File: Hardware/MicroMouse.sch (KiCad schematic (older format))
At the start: 74 parts, among them J1 TSW-106-25-S-S-RA, J2 B2B-PH-K-S(LF)(SN), J3 Conn_01x04_Male, J4 B5B-XH-A(LF)(SN), J5 B5B-XH-A(LF)(SN), Q1 NXV75UPR, SW1 SPST, SW2 SPST, SW3 SPST, SW4 SPST, SW6 SPST, SW7 SPST, SW8 SPST, U1 ADP1612, U2 PIC16F886-E_SO, U3 ULN2803ADW, U4 74LVC1G332GV-Q100H, U5 ADCMP393ARZ, U6 TCRT1000, U7 TCRT1000, U8 TCRT1000, Y1 32.768KHZ

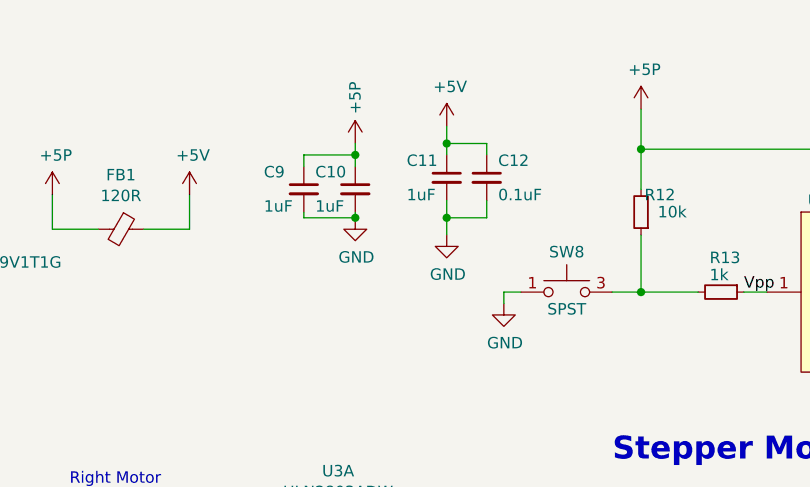
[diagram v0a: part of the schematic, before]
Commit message: Layout
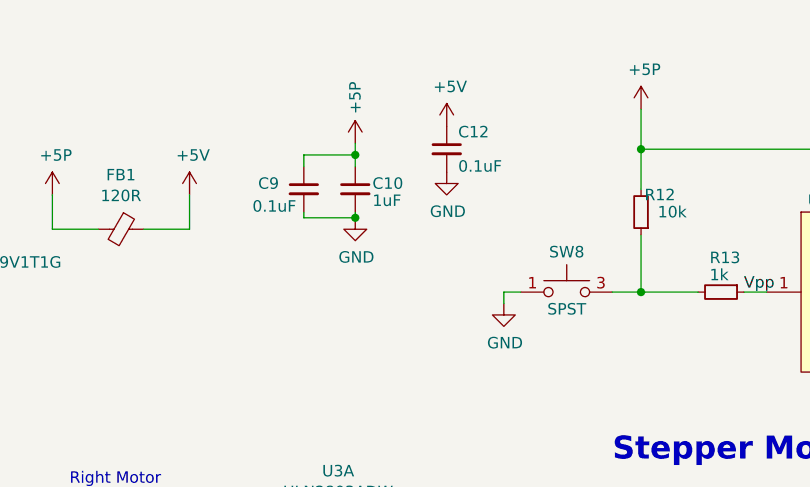
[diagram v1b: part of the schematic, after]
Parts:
- removed C11: 1uF, Micro-Footprint:CAP0603, symbol Device:C_Small
- C9: value 1uF -> 0.1uF
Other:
- moved on the sheet: C12
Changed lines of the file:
@@
 	10025 1875 10025 1950
-$Comp
-L Device:C_Small C11
-U 1 1 607C5E25
-P 5725 1275
-F 0 "C11" H 5550 1350 50  0000 L CNN
-F 1 "1uF" H 5550 1200 50  0000 L CNN
-F 2 "Micro-Footprint:CAP0603" H 5725 1275 50  0001 C CNN
-F 3 "~" H 5725 1275 50  0001 C CNN
-	1    5725 1275
-	1    0    0    -1
-$EndComp
 $Comp
 L Device:C_Small C12
 U 1 1 607C6AE3
-P 5900 1275
-F 0 "C12" H 5950 1350 50  0000 L CNN
-F 1 "0.1uF" H 5950 1200 50  0000 L CNN
-F 2 "Micro-Footprint:CAP0603" H 5900 1275 50  0001 C CNN
-F 3 "~" H 5900 1275 50  0001 C CNN
-	1    5900 1275
+P 5725 1150
+F 0 "C12" H 5775 1225 50  0000 L CNN
+F 1 "0.1uF" H 5775 1075 50  0000 L CNN
+F 2 "Micro-Footprint:CAP0603" H 5725 1150 50  0001 C CNN
+F 3 "~" H 5725 1150 50  0001 C CNN
+	1    5725 1150
 	1    0    0    -1
 $EndComp
@@
 	1    0    0    -1
 $EndComp
-Wire Wire Line
-	5725 1175 5725 1125
-Wire Wire Line
-	5900 1175 5900 1125
-Wire Wire Line
-	5900 1125 5725 1125
-Connection ~ 5725 1125
-Wire Wire Line
-	5725 1125 5725 1050
 $Comp
 L power:GND #PWR021
 U 1 1 607CD1DE
-P 5725 1525
-F 0 "#PWR021" H 5725 1275 50  0001 C CNN
-F 1 "GND" H 5730 1352 50  0000 C CNN
-F 2 "" H 5725 1525 50  0001 C CNN
-F 3 "" H 5725 1525 50  0001 C CNN
-	1    5725 1525
+P 5725 1250
+F 0 "#PWR021" H 5725 1000 50  0001 C CNN
+F 1 "GND" H 5730 1077 50  0000 C CNN
+F 2 "" H 5725 1250 50  0001 C CNN
+F 3 "" H 5725 1250 50  0001 C CNN
+	1    5725 1250
 	1    0    0    -1
 $EndComp
@@
 	9350 3275 9400 3275
 $Comp
-L Device:C_Small C9
-U 1 1 607C4D9D
-P 5100 1325
-F 0 "C9" H 4925 1400 50  0000 L CNN
-F 1 "1uF" H 4925 1250 50  0000 L CNN
-F 2 "Micro-Footprint:CAP0603" H 5100 1325 50  0001 C CNN
-F 3 "~" H 5100 1325 50  0001 C CNN
-	1    5100 1325
-	1    0    0    -1
-$EndComp
-$Comp
 L Device:C_Small C10
 U 1 1 607C5B06
 P 5325 1325
-F 0 "C10" H 5150 1400 50  0000 L CNN
-F 1 "1uF" H 5150 1250 50  0000 L CNN
+F 0 "C10" H 5400 1350 50  0000 L CNN
+F 1 "1uF" H 5400 1275 50  0000 L CNN
 F 2 "Micro-Footprint:CAP0603" H 5325 1325 50  0001 C CNN
 F 3 "~" H 5325 1325 50  0001 C CNN
@@
 Wire Wire Line
 	6450 5525 6450 5500
-Wire Wire Line
-	5725 1525 5725 1450
-Wire Wire Line
-	5900 1375 5900 1450
-Wire Wire Line
-	5900 1450 5725 1450
-Connection ~ 5725 1450
-Wire Wire Line
-	5725 1450 5725 1375
 Wire Wire Line
 	1650 6275 1650 6225
@@
 	3275 2250 3275 2225
 $Comp
-L power:GND #PWR?
+L power:GND #PWR0108
 U 1 1 6137EB99
 P 4500 3750
-F 0 "#PWR?" H 4500 3500 50  0001 C CNN
+F 0 "#PWR0108" H 4500 3500 50  0001 C CNN
 F 1 "GND" H 4505 3577 50  0000 C CNN
 F 2 "" H 4500 3750 50  0001 C CNN
@@
 	4500 3750 4500 3600
 $Comp
-L power:GND #PWR?
+L power:GND #PWR0109
 U 1 1 613AB2FA
 P 9400 3575
-F 0 "#PWR?" H 9400 3325 50  0001 C CNN
+F 0 "#PWR0109" H 9400 3325 50  0001 C CNN
 F 1 "GND" H 9400 3425 50  0000 C CNN
 F 2 "" H 9400 3575 50  0001 C CNN
@@
 Wire Wire Line
 	9400 3575 9400 3525
+$Comp
+L Device:C_Small C9
+U 1 1 60D66234
+P 5100 1325
+F 0 "C9" H 4900 1350 50  0000 L CNN
+F 1 "0.1uF" H 4875 1250 50  0000 L CNN
+F 2 "Micro-Footprint:CAP0603" H 5100 1325 50  0001 C CNN
+F 3 "~" H 5100 1325 50  0001 C CNN
+	1    5100 1325
+	1    0    0    -1
+$EndComp
 $EndSCHEMATC
